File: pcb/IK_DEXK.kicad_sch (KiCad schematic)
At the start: 11 parts, among them SW1 SW_Push, SW2 SW_Push, SW3 SW_Push, SW4 SW_Push, SW5 SW_Push, SW6 SW_Push, SW7 SW_Push, SW8 SW_Push, SW9 SW_Push, U1 MOUDLE-SEEEDUINO-XIAO, U2 ER_OLEDM0.91_1x-I2C

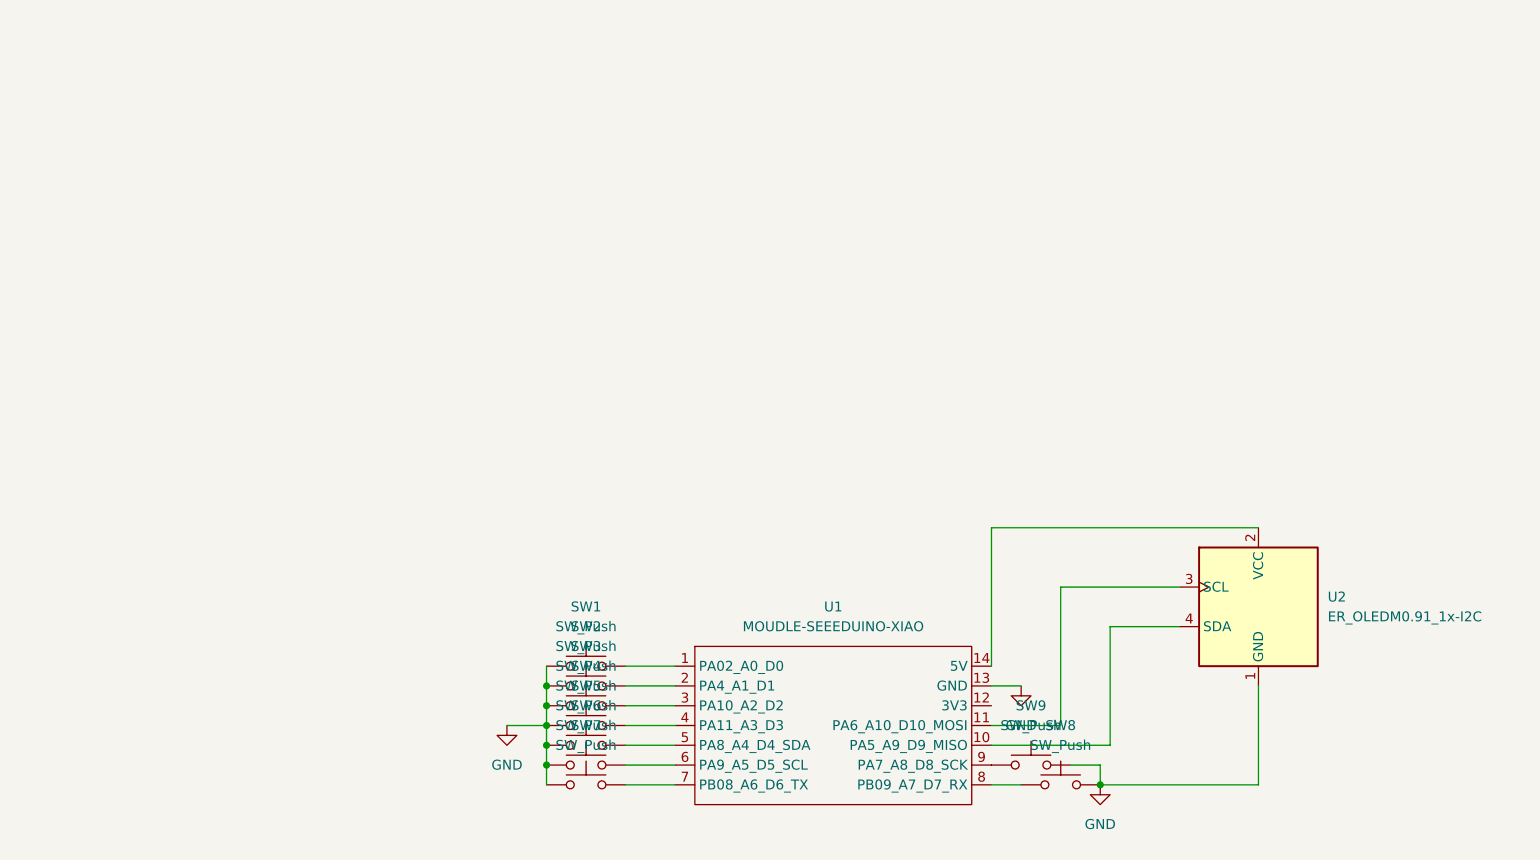
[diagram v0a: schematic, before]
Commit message: everything
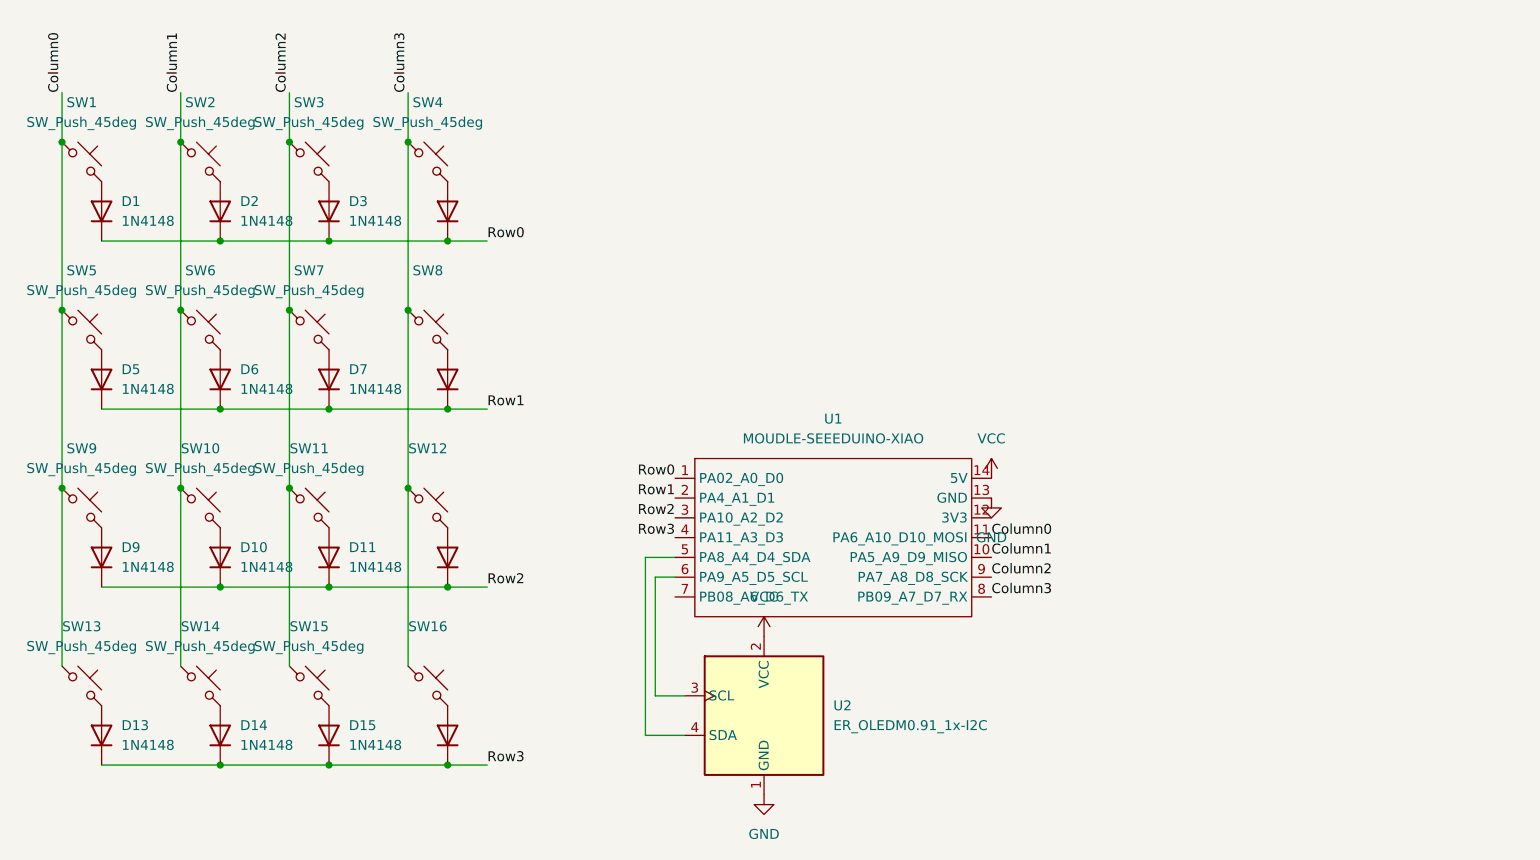
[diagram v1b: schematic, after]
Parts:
- removed SW1, SW2, SW3, SW4, SW5, SW6, SW7, SW8, SW9: SW_Push, Button_Switch_Keyboard:SW_Cherry_MX_1.00u_PCB, symbol Switch:SW_Push
- added D1, D10, D11, D12, D13, D14, D15, D16, D2, D3, D4, D5, D6, D7, D8, D9: 1N4148, Diode_THT:D_DO-35_SOD27_P7.62mm_Horizontal, symbol Diode:1N4148
- added SW1, SW10, SW11, SW12, SW13, SW14, SW15, SW16, SW2, SW3, SW4, SW5, SW6, SW7, SW8, SW9: SW_Push_45deg, Button_Switch_Keyboard:SW_Cherry_MX_1.00u_PCB, symbol Switch:SW_Push_45deg
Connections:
- net Row1: now reaches U1.2 (PA4_A1_D1)
- net Row1: now also D5.1 (K), D6.1 (K), D7.1 (K), D8.1 (K)
- net Row0: now reaches U1.1 (PA02_A0_D0)
- net Row0: now also D1.1 (K), D2.1 (K), D3.1 (K), D4.1 (K)
- net at U2.4 (SDA): now also U1.5 (PA8_A4_D4_SDA); no longer U1.10 (PA5_A9_D9_MISO)
- net at U2.3 (SCL): now also U1.6 (PA9_A5_D5_SCL); no longer U1.11 (PA6_A10_D10_MOSI)
- net VCC: now reaches U1.14 (5V), U2.2 (VCC)
- net Row2: now reaches U1.3 (PA10_A2_D2)
- net Row2: now also D10.1 (K), D11.1 (K), D12.1 (K), D9.1 (K)
- net Row3: now reaches U1.4 (PA11_A3_D3)
- net Row3: now also D13.1 (K), D14.1 (K), D15.1 (K), D16.1 (K)
- net Column3: now reaches U1.8 (PB09_A7_D7_RX)
- net Column3: now also SW12.1, SW16.1, SW4.1, SW8.1
- net Column2: now reaches U1.9 (PA7_A8_D8_SCK)
- net Column2: now also SW11.1, SW15.1, SW3.1, SW7.1
- new net: D8.2 (A), SW8.2
- new net: D12.2 (A), SW12.2
- new net: D2.2 (A), SW2.2
- new net: D3.2 (A), SW3.2
- new net: D11.2 (A), SW11.2
- new net: D6.2 (A), SW6.2
- new net: D10.2 (A), SW10.2
- new net: D4.2 (A), SW4.2
- new net: D5.2 (A), SW5.2
- new net: D1.2 (A), SW1.2
- new net: D7.2 (A), SW7.2
- new net: D13.2 (A), SW13.2
- new net: D16.2 (A), SW16.2
- new net: D14.2 (A), SW14.2
- new net: D15.2 (A), SW15.2
- new net: D9.2 (A), SW9.2
- new net Column0: SW1.1, SW13.1, SW5.1, SW9.1, U1.11 (PA6_A10_D10_MOSI)
- new net Column1: SW10.1, SW14.1, SW2.1, SW6.1, U1.10 (PA5_A9_D9_MISO)
